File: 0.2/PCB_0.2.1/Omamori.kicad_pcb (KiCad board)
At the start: 2 copper layers, 25 x 35 mm, 29 parts, among them J1 Conn_01x04_Female, U1 BQ25504, U2 TPS61222DCK, U3 ATtiny85, U4 TS-1233

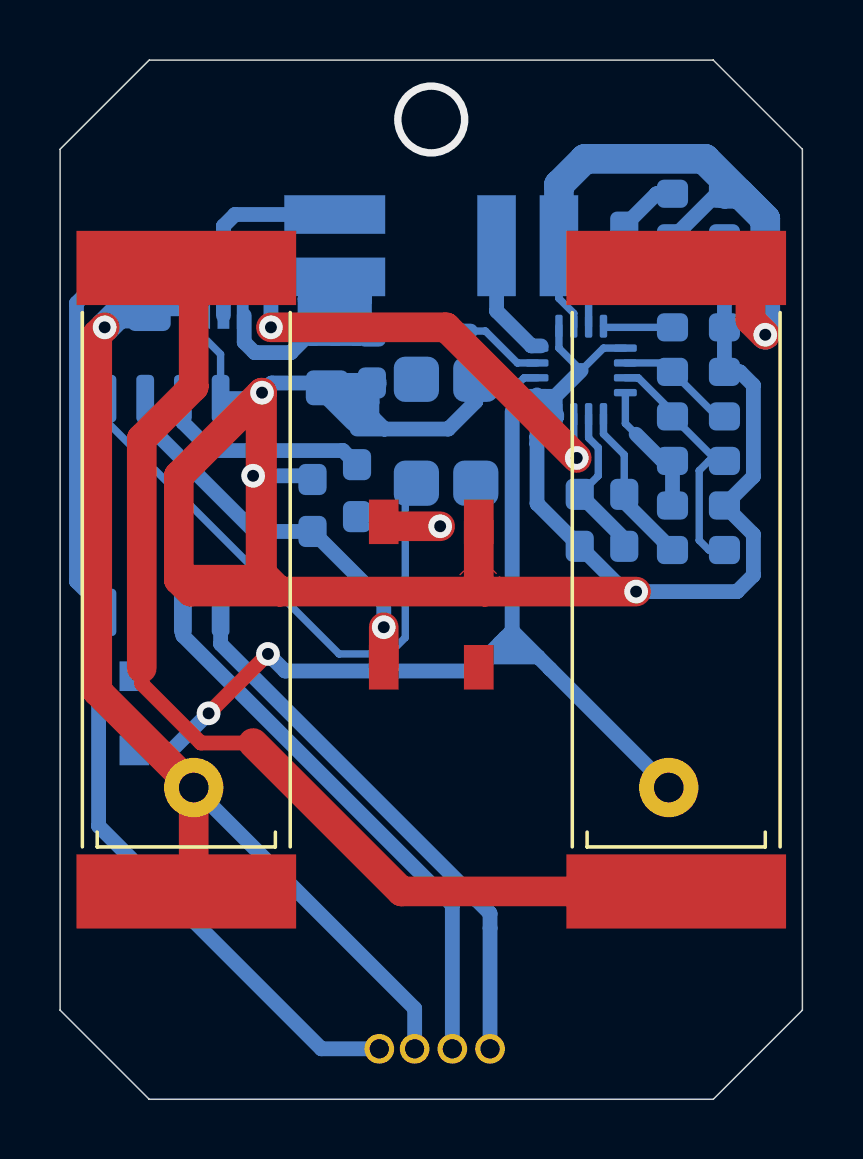
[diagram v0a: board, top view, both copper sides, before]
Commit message: Updated 0.2.1 PCB design.
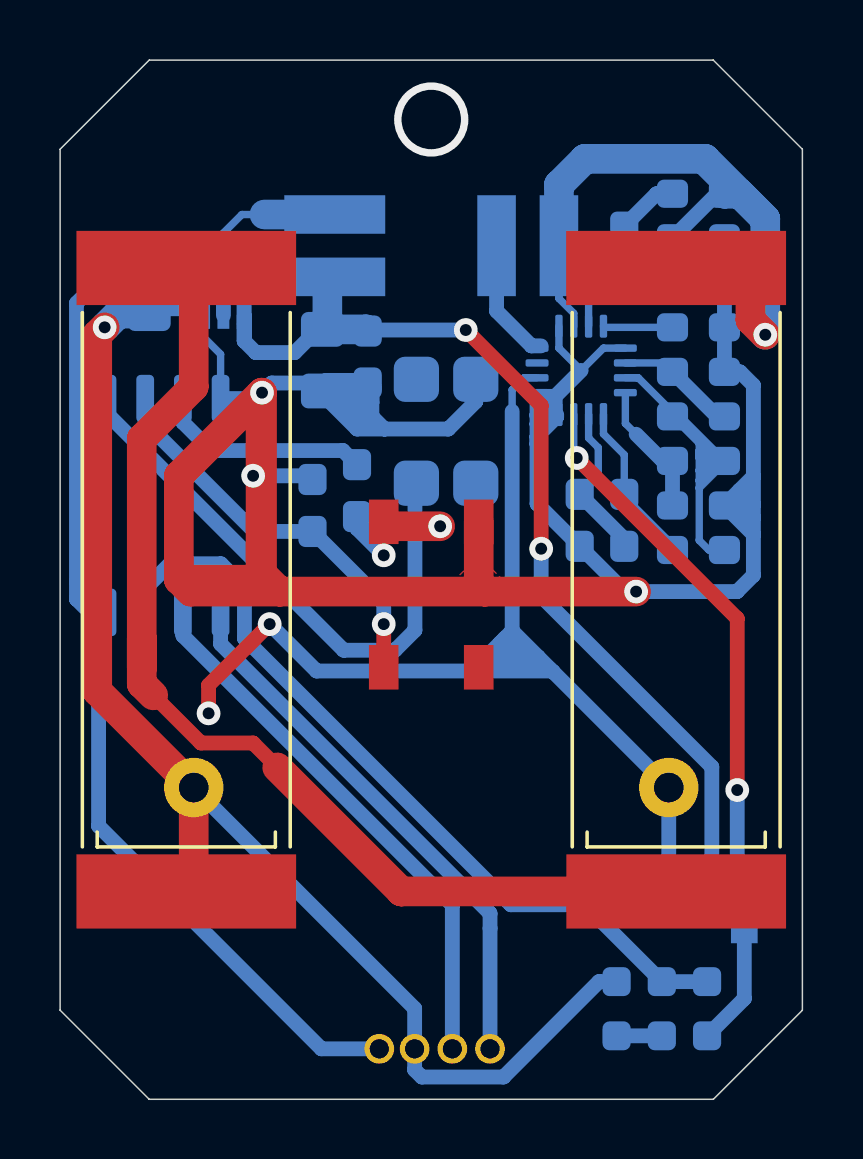
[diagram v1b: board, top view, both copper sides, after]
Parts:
- removed D2: DIODE, Diode_SMD:D_SOD-323_HandSoldering
- added Q1: IRLML0030, Package_TO_SOT_SMD:SOT-23, B.Cu at (34.5, 40.9)
- added R_oc3: 1.8M, Resistor_SMD:R_0603_1608Metric_Pad0.98x0.95mm_HandSolder, B.Cu at (34.3, 44.5)
- added R_oc4: 8.2M, Resistor_SMD:R_0603_1608Metric_Pad0.98x0.95mm_HandSolder, B.Cu at (32.8, 44.5)
- added R_oc5: 10M, Resistor_SMD:R_0603_1608Metric_Pad0.98x0.95mm_HandSolder, B.Cu at (31.2, 44.5)
- moved C_pre_boost1 0.20 mm to (21.3, 22.6)
- moved C_filter1 0.14 mm to (22.9, 22.5)
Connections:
- C_filter1 pad 1: /Vstor -> Net-(C_filter1-Pad1)
- C_pre_boost1 pad 1: /Vstor -> Net-(C_filter1-Pad1)
- L_boost1 pad 1: /Vstor -> Net-(C_filter1-Pad1)
- U1 pad 15: /Vstor -> (no net)
- U2 pad 1: /Vstor -> Net-(C_filter1-Pad1)
- U2 pad 6: /Vbat_ok -> Net-(C_filter1-Pad1)
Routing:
- net Net-(C_filter1-Pad1): track 0.00 -> 42.2 mm, vias 0 -> 2
- net /Vmeasure: track 2.30 -> 27.4 mm
- net /Vstor: track 21.1 -> 0.00 mm
- net GND: track 132.7 -> 146.5 mm
- net /Vr_div: track 8.90 -> 16.1 mm
- net Net-(C_super1-Pad1): track 34.1 -> 39.8 mm
- net Net-(Sol_1-Pad2): track 35.6 -> 38.9 mm
- net /Din_LED: track 2.01 -> 4.82 mm, vias 1 -> 2
- net Net-(R_oc4-Pad1): track 0.00 -> 1.52 mm
- net /Vbat_ok: track 16.7 -> 17.9 mm
- net /Vcc_ATTiny: track 39.2 -> 39.9 mm
